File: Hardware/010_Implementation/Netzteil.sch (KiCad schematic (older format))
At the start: 5 parts, among them U1 LT1086-5.0

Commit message: Board version 4
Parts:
- removed U1: LT1086-5.0, Board:DPAK254P1394X457-4N, symbol Regulator_Linear:LT1086-5.0
- added C3: 22u, Capacitor_SMD:C_0603_1608Metric_Pad1.05x0.95mm_HandSolder, symbol Device:C
- added L1: 2.2u, Capacitor_SMD:C_0603_1608Metric_Pad1.05x0.95mm_HandSolder, symbol Device:L
- added R3: 100k, Resistor_SMD:R_0805_2012Metric_Pad1.15x1.40mm_HandSolder, symbol Device:R
- added U1: TPS62163DGK, Package_SO:VSSOP-8_3.0x3.0mm_P0.65mm, symbol Regulator_Switching:TPS62163DSG
- C1: footprint Capacitor_SMD:C_1812_4532Metric_Pad1.30x3.40mm_HandSolder -> Capacitor_SMD:C_0603_1608Metric_Pad1.05x0.95mm_HandSolder
- C2: value 100n -> 10u; footprint Capacitor_SMD:C_1812_4532Metric_Pad1.30x3.40mm_HandSolder -> Capacitor_SMD:C_0603_1608Metric_Pad1.05x0.95mm_HandSolder
- R1: value 1k -> 10k
- R2: value 100 -> 1k
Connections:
- wire segments 22 -> 44
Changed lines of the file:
@@
 Text Notes 4175 2300 2    50   ~ 0
 12V-OBD Power Supply
-Wire Wire Line
-	6850 2825 6850 2875
-Wire Wire Line
-	6850 3175 6850 3225
-$Comp
-L Device:C C2
-U 1 1 5F6089EB
-P 6850 3025
-F 0 "C2" H 6965 3071 50  0000 L CNN
-F 1 "100n" H 6965 2980 50  0000 L CNN
-F 2 "Capacitor_SMD:C_1812_4532Metric_Pad1.30x3.40mm_HandSolder" H 6888 2875 50  0001 C CNN
-F 3 "~" H 6850 3025 50  0001 C CNN
-	1    6850 3025
-	1    0    0    -1
-$EndComp
-Wire Wire Line
-	6850 2825 7025 2825
-$Comp
-L power:GND #PWR02
-U 1 1 5FA1043A
-P 7950 3300
-F 0 "#PWR02" H 7950 3050 50  0001 C CNN
-F 1 "GND" H 7955 3127 50  0000 C CNN
-F 2 "" H 7950 3300 50  0001 C CNN
-F 3 "" H 7950 3300 50  0001 C CNN
-	1    7950 3300
-	1    0    0    -1
-$EndComp
-Wire Wire Line
-	7950 3225 7950 3300
-Wire Wire Line
-	6850 2825 6775 2825
-Connection ~ 6850 2825
-Wire Wire Line
-	7625 2825 7950 2825
-$Comp
-L Regulator_Linear:LT1086-5.0 U1
-U 1 1 5FA0C017
-P 7325 2825
-F 0 "U1" H 7325 3067 50  0000 C CNN
-F 1 "LT1086-5.0" H 7325 2976 50  0000 C CNN
-F 2 "Board:DPAK254P1394X457-4N" H 7325 3075 50  0001 C CIN
-F 3 "https://www.analog.com/media/en/technical-documentation/data-sheets/1086ffs.pdf" H 7325 2825 50  0001 C CNN
-	1    7325 2825
-	1    0    0    -1
-$EndComp
-Wire Wire Line
-	6850 3225 7325 3225
-Wire Wire Line
-	7325 3125 7325 3225
-Connection ~ 7325 3225
-Wire Wire Line
-	7325 3225 7950 3225
 $Comp
 L Device:R R1
@@
 P 5025 3425
 F 0 "R1" H 5095 3471 50  0000 L CNN
-F 1 "1k" H 5095 3380 50  0000 L CNN
+F 1 "10k" H 5095 3380 50  0000 L CNN
 F 2 "Resistor_SMD:R_0805_2012Metric_Pad1.15x1.40mm_HandSolder" V 4955 3425 50  0001 C CNN
 F 3 "~" H 5025 3425 50  0001 C CNN
@@
 P 5025 3875
 F 0 "R2" H 5095 3921 50  0000 L CNN
-F 1 "100" H 5095 3830 50  0000 L CNN
+F 1 "1k" H 5095 3830 50  0000 L CNN
 F 2 "Resistor_SMD:R_0805_2012Metric_Pad1.15x1.40mm_HandSolder" V 4955 3875 50  0001 C CNN
 F 3 "~" H 5025 3875 50  0001 C CNN
@@
 L power:PWR_FLAG #FLG01
 U 1 1 5FB093DE
-P 6775 2825
-F 0 "#FLG01" H 6775 2900 50  0001 C CNN
-F 1 "PWR_FLAG" H 6775 2998 50  0000 C CNN
-F 2 "" H 6775 2825 50  0001 C CNN
-F 3 "~" H 6775 2825 50  0001 C CNN
-	1    6775 2825
-	1    0    0    -1
-$EndComp
-Connection ~ 6775 2825
-Wire Wire Line
-	6775 2825 5025 2825
+P 5425 2825
+F 0 "#FLG01" H 5425 2900 50  0001 C CNN
+F 1 "PWR_FLAG" H 5425 2998 50  0000 C CNN
+F 2 "" H 5425 2825 50  0001 C CNN
+F 3 "~" H 5425 2825 50  0001 C CNN
+	1    5425 2825
+	1    0    0    -1
+$EndComp
 $Comp
 L Device:C C1
@@
 F 0 "C1" H 4765 3921 50  0000 L CNN
 F 1 "10n" H 4765 3830 50  0000 L CNN
-F 2 "Capacitor_SMD:C_1812_4532Metric_Pad1.30x3.40mm_HandSolder" H 4688 3725 50  0001 C CNN
+F 2 "Capacitor_SMD:C_0603_1608Metric_Pad1.05x0.95mm_HandSolder" H 4688 3725 50  0001 C CNN
 F 3 "~" H 4650 3875 50  0001 C CNN
 	1    4650 3875
@@
 	4850 4150 4650 4150
 $Comp
-L power:+5V #PWR021
+L power:+5V #PWR05
 U 1 1 5FA170AE
-P 7950 2825
-F 0 "#PWR021" H 7950 2675 50  0001 C CNN
-F 1 "+5V" H 7965 2998 50  0000 C CNN
-F 2 "" H 7950 2825 50  0001 C CNN
-F 3 "" H 7950 2825 50  0001 C CNN
-	1    7950 2825
-	1    0    0    -1
-$EndComp
+P 10625 2750
+F 0 "#PWR05" H 10625 2600 50  0001 C CNN
+F 1 "+5V" H 10640 2923 50  0000 C CNN
+F 2 "" H 10625 2750 50  0001 C CNN
+F 3 "" H 10625 2750 50  0001 C CNN
+	1    10625 2750
+	1    0    0    -1
+$EndComp
+Connection ~ 5425 2825
+Wire Wire Line
+	5425 2825 5025 2825
+Wire Wire Line
+	5425 2825 6975 2825
+$Comp
+L Regulator_Switching:TPS62163DSG U1
+U 1 1 5FB37DEF
+P 7975 3125
+F 0 "U1" H 7975 3692 50  0000 C CNN
+F 1 "TPS62163DGK" H 7975 3601 50  0000 C CNN
+F 2 "Package_SO:VSSOP-8_3.0x3.0mm_P0.65mm" H 8125 2775 50  0001 L CNN
+F 3 "http://www.ti.com/lit/ds/symlink/tps62160.pdf" H 7975 3675 50  0001 C CNN
+	1    7975 3125
+	1    0    0    -1
+$EndComp
+$Comp
+L Device:L L1
+U 1 1 5FB3AA0A
+P 8650 2825
+F 0 "L1" V 8840 2825 50  0000 C CNN
+F 1 "2.2u" V 8749 2825 50  0000 C CNN
+F 2 "Capacitor_SMD:C_0603_1608Metric_Pad1.05x0.95mm_HandSolder" H 8650 2825 50  0001 C CNN
+F 3 "~" H 8650 2825 50  0001 C CNN
+	1    8650 2825
+	0    -1   -1   0
+$EndComp
+$Comp
+L Device:R R3
+U 1 1 5FB3B31A
+P 8250 4225
+F 0 "R3" V 8043 4225 50  0000 C CNN
+F 1 "100k" V 8134 4225 50  0000 C CNN
+F 2 "Resistor_SMD:R_0805_2012Metric_Pad1.15x1.40mm_HandSolder" V 8180 4225 50  0001 C CNN
+F 3 "~" H 8250 4225 50  0001 C CNN
+	1    8250 4225
+	0    1    1    0
+$EndComp
+Wire Wire Line
+	8375 2825 8500 2825
+Wire Wire Line
+	8800 2825 8925 2825
+Wire Wire Line
+	7575 3225 7575 4225
+Wire Wire Line
+	7575 4225 8100 4225
+Wire Wire Line
+	8925 4225 8925 2925
+Connection ~ 8925 2825
+Wire Wire Line
+	8400 4225 8925 4225
+$Comp
+L power:GND #PWR03
+U 1 1 5FB3F4B3
+P 7975 3750
+F 0 "#PWR03" H 7975 3500 50  0001 C CNN
+F 1 "GND" H 7980 3577 50  0000 C CNN
+F 2 "" H 7975 3750 50  0001 C CNN
+F 3 "" H 7975 3750 50  0001 C CNN
+	1    7975 3750
+	1    0    0    -1
+$EndComp
+Wire Wire Line
+	7975 3750 7975 3575
+Wire Wire Line
+	8075 3575 8075 3525
+Connection ~ 7975 3575
+Wire Wire Line
+	7975 3575 8075 3575
+Wire Wire Line
+	7975 3525 7975 3575
+Wire Wire Line
+	8375 2925 8925 2925
+Connection ~ 8925 2925
+Wire Wire Line
+	8925 2925 8925 2825
+$Comp
+L Device:C C2
+U 1 1 5FB43F56
+P 6975 3100
+F 0 "C2" H 7090 3146 50  0000 L CNN
+F 1 "10u" H 7090 3055 50  0000 L CNN
+F 2 "Capacitor_SMD:C_0603_1608Metric_Pad1.05x0.95mm_HandSolder" H 7013 2950 50  0001 C CNN
+F 3 "~" H 6975 3100 50  0001 C CNN
+	1    6975 3100
+	1    0    0    -1
+$EndComp
+Wire Wire Line
+	7575 2925 7450 2925
+Wire Wire Line
+	7450 2925 7450 2825
+Connection ~ 7450 2825
+Wire Wire Line
+	7450 2825 7575 2825
+Wire Wire Line
+	6975 2950 6975 2825
+Connection ~ 6975 2825
+Wire Wire Line
+	6975 2825 7450 2825
+$Comp
+L power:GND #PWR02
+U 1 1 5FB459AA
+P 6975 3425
+F 0 "#PWR02" H 6975 3175 50  0001 C CNN
+F 1 "GND" H 6980 3252 50  0000 C CNN
+F 2 "" H 6975 3425 50  0001 C CNN
+F 3 "" H 6975 3425 50  0001 C CNN
+	1    6975 3425
+	1    0    0    -1
+$EndComp
+Wire Wire Line
+	6975 3425 6975 3250
+$Comp
+L power:GND #PWR04
+U 1 1 5FB4620B
+P 9975 3500
+F 0 "#PWR04" H 9975 3250 50  0001 C CNN
+F 1 "GND" H 9980 3327 50  0000 C CNN
+F 2 "" H 9975 3500 50  0001 C CNN
+F 3 "" H 9975 3500 50  0001 C CNN
+	1    9975 3500
+	1    0    0    -1
+$EndComp
+Wire Wire Line
+	10625 2825 10625 2750
+$Comp
+L Device:C C3
+U 1 1 5FB437F9
+P 9975 3025
+F 0 "C3" H 10090 3071 50  0000 L CNN
+F 1 "22u" H 10090 2980 50  0000 L CNN
+F 2 "Capacitor_SMD:C_0603_1608Metric_Pad1.05x0.95mm_HandSolder" H 10013 2875 50  0001 C CNN
+F 3 "~" H 9975 3025 50  0001 C CNN
+	1    9975 3025
+	1    0    0    -1
+$EndComp
+Wire Wire Line
+	8925 2825 9975 2825
+Wire Wire Line
+	9975 2875 9975 2825
+Connection ~ 9975 2825
+Wire Wire Line
+	9975 2825 10450 2825
+Wire Wire Line
+	9975 3275 9525 3275
+Wire Wire Line
+	9525 3275 9525 3025
+Wire Wire Line
+	9525 3025 8375 3025
+Wire Wire Line
+	9975 3175 9975 3275
+Wire Wire Line
+	9975 3275 9975 3500
+Connection ~ 9975 3275
+$Comp
+L power:PWR_FLAG #FLG02
+U 1 1 5FB4D740
+P 10450 2825
+F 0 "#FLG02" H 10450 2900 50  0001 C CNN
+F 1 "PWR_FLAG" H 10450 2998 50  0000 C CNN
+F 2 "" H 10450 2825 50  0001 C CNN
+F 3 "~" H 10450 2825 50  0001 C CNN
+	1    10450 2825
+	1    0    0    -1
+$EndComp
+Connection ~ 10450 2825
+Wire Wire Line
+	10450 2825 10625 2825
+Wire Wire Line
+	7875 3525 7875 3575
+Wire Wire Line
+	7875 3575 7975 3575
 $EndSCHEMATC

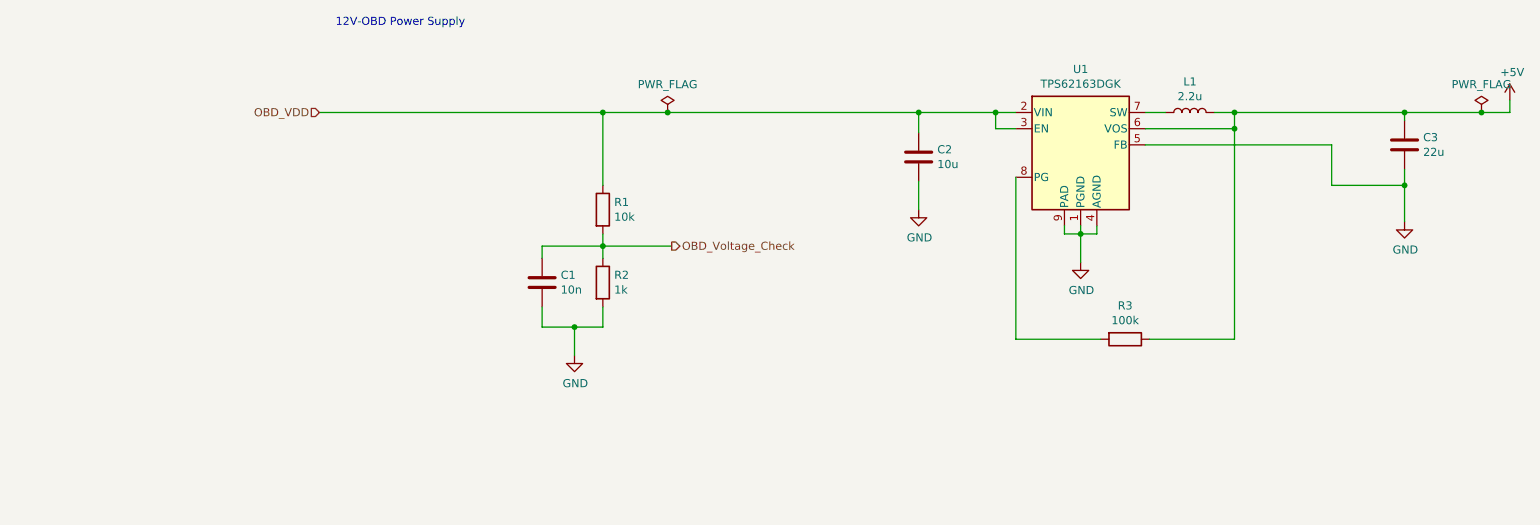
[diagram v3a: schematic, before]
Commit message: Board Version 4.2
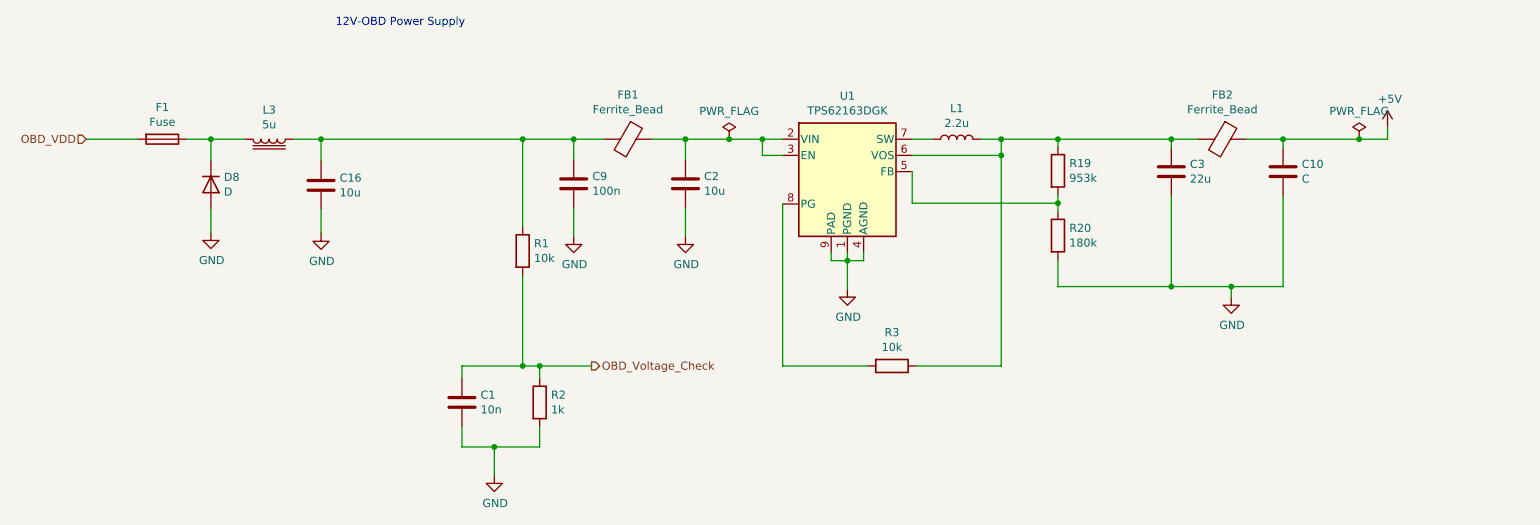
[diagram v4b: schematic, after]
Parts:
- added C10: C, symbol Device:C
- added C16: 10u, symbol Device:C
- added C9: 100n, Capacitor_SMD:C_0603_1608Metric_Pad1.05x0.95mm_HandSolder, symbol Device:C
- added D8: D, symbol Device:D
- added F1: Fuse, symbol Device:Fuse
- added FB1, FB2: Ferrite_Bead, symbol Device:Ferrite_Bead
- added L3: 5u, symbol Device:L_Core_Iron
- added R19: 953k, symbol Device:R
- added R20: 180k, symbol Device:R
- R3: value 100k -> 10k
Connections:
- net +5V: now also C10.1, FB2.1; no longer C3.1, L1.2, R3.1, U1.6 (VOS)
- net GND: now also C10.2, C16.2, C9.2, D8.2 (A), R20.2; no longer U1.5 (FB)
- net OBD_VDD: now also F1.2; no longer C2.1, R1.1, U1.2 (VIN), U1.3 (EN)
- new net: C3.1, FB2.2, L1.2, R19.1, R3.1, U1.6 (VOS)
- new net: R19.2, R20.1, U1.5 (FB)
- new net: C16.1, C9.1, FB1.2, L3.1, R1.1
- new net: C2.1, FB1.1, U1.2 (VIN), U1.3 (EN)
- new net: D8.1 (K), F1.1, L3.2
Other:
- moved on the sheet: C1, C2, C3, L1, R1, R2, R3, U1
